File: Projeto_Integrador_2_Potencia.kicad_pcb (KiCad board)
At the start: 2 copper layers, 150 x 100 mm, 17 parts, among them J10 Borne_CMD_Interface, J2 Vi 24V, J3 Vo 48V, J4 INA219_01x02_Socket_3.5mm, J5 INA219_01x06_Socket_2.55mm, J7 Display_01x04_Socket, J9 PWM_Connector, Q1 IRF740, U1 ESP32-DEVKIT-V1

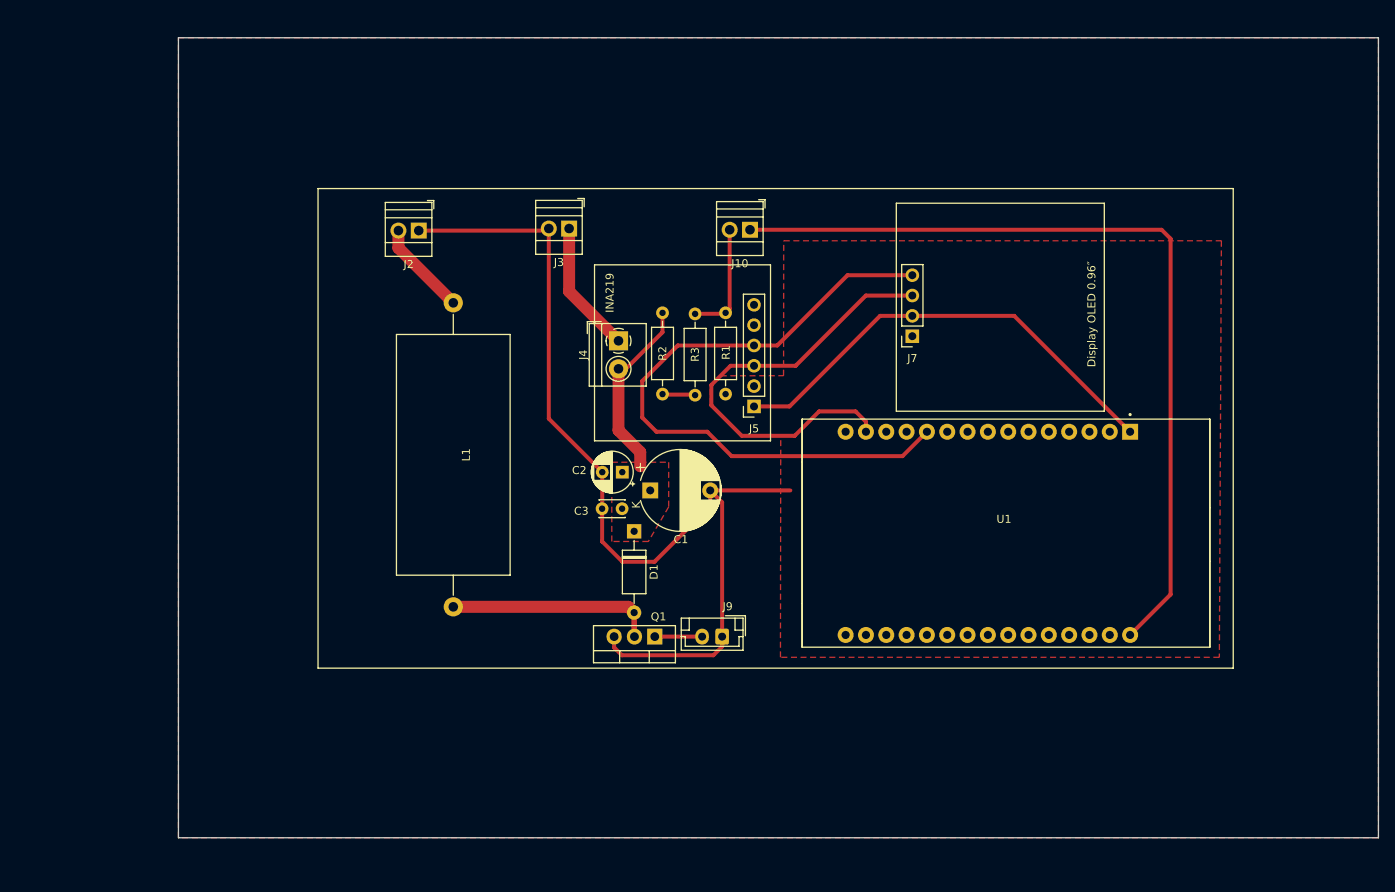
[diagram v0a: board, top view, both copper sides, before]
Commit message: Mudanças após primeira manufatura
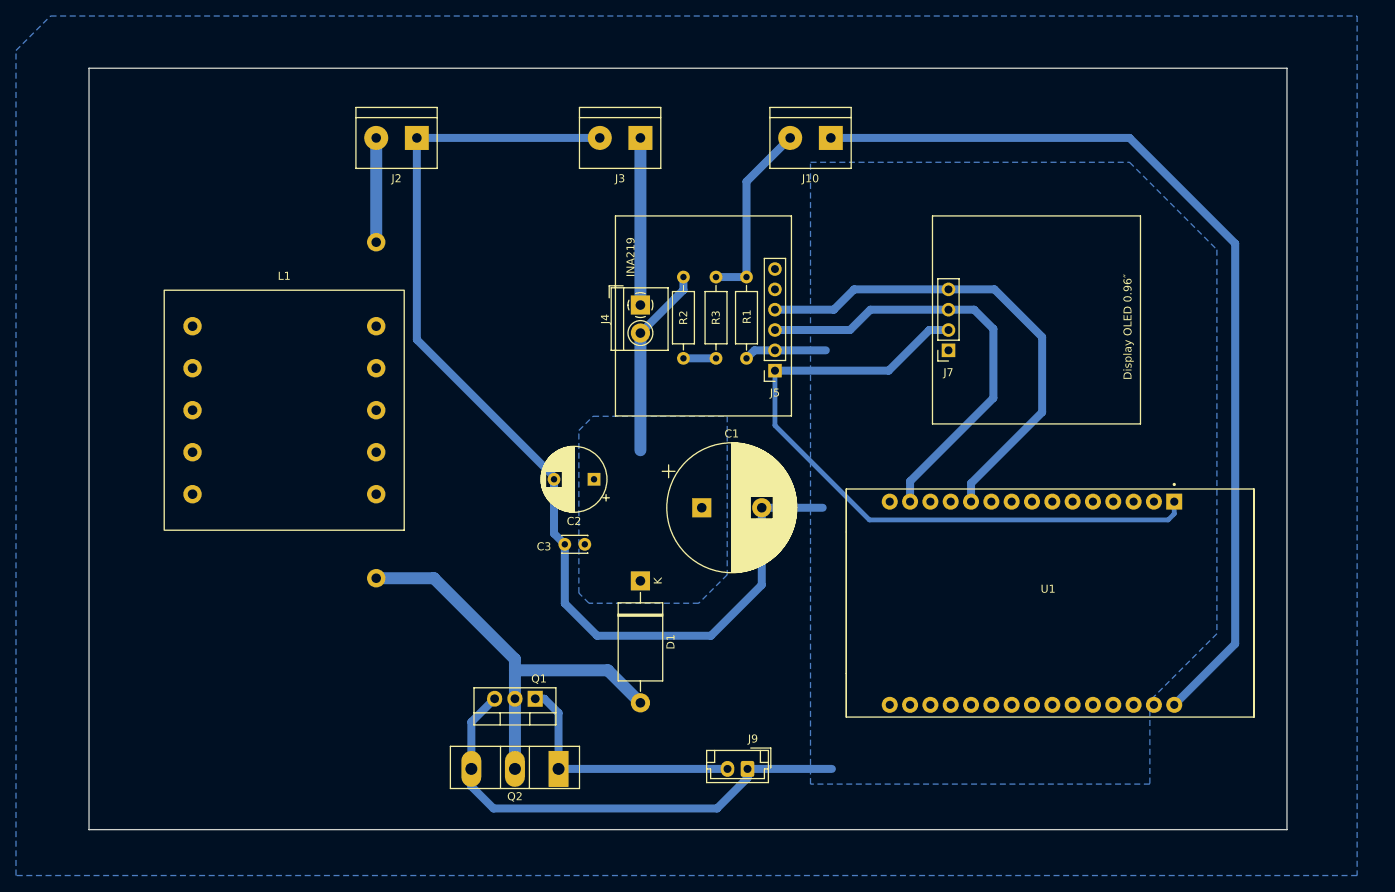
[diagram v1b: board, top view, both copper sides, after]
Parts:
- added Q2: 47N60, Package_TO_SOT_THT:TO-247-3_Vertical, F.Cu at (112.0, 137.3)
- C1: footprint Capacitor_THT:CP_Radial_D10.0mm_P7.50mm -> Capacitor_THT:CP_Radial_D16.0mm_P7.50mm
- C2: footprint Capacitor_THT:CP_Radial_D5.0mm_P2.50mm -> Capacitor_THT:CP_Radial_D8.0mm_P5.00mm
- D1: value ~ -> Diodo Schottky; footprint Diode_THT:D_A-405_P10.16mm_Horizontal -> Diode_THT:D_DO-27_P15.24mm_Horizontal
- J10, J2, J3: footprint TerminalBlock:TerminalBlock_Xinya_XY308-2.54-2P_1x02_P2.54mm_Horizontal -> TerminalBlock:TerminalBlock_bornier-2_P5.08mm
- L1: footprint Inductor_THT:L_Axial_L29.9mm_D14.0mm_P38.00mm_Horizontal_Vishay_IHA-105 -> Integrador_2:Indutor_Integrador_2
- moved L1 25.0 mm to (77.7, 92.5), turned to 180 degrees
- moved J9 16.8 mm to (135.6, 137.3)
- moved Q1 16.8 mm to (109.1, 128.5)
- moved J10 15.3 mm to (146.1, 58.4)
- moved J3 14.4 mm to (122.2, 58.4)
- moved J2 11.6 mm to (94.3, 58.4)
- moved U1 10.3 mm to (173.5, 116.6)
- moved C1 6.79 mm to (129.9, 104.6)
- moved C3 6.45 mm to (115.3, 109.2)
- moved D1 6.25 mm to (122.2, 113.8)
- moved R3 5.30 mm to (131.7, 86.0)
- moved J4 5.24 mm to (122.2, 79.3)
- moved R1 5.18 mm to (135.5, 75.8)
- moved R2 5.18 mm to (127.6, 75.8)
- moved J5 5.18 mm to (139.1, 87.5)
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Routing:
- net GND: track 123.5 -> 206.3 mm
- net 3V3: track 57.6 -> 87.3 mm
- net pwm: track 5.92 -> 31.8 mm
- net Net-(D1-A): track 27.4 -> 52.6 mm
- net I2C_Sda: track 82.6 -> 61.2 mm
- net 8V: track 104.7 -> 116.8 mm
- net 5.2V_feedback: track 14.5 -> 23.5 mm
- net INA_Vin+: track 16.6 -> 20.9 mm
- net Net-(J2-Pin_2): track 11.9 -> 13.0 mm
- net I2C_Scl: track 56.2 -> 55.3 mm
- net INA_Vin-: track 23.1 -> 23.9 mm
- added copper zone on B.Cu, net (none)
- added copper zone on B.Cu, net GND
- added copper zone on B.Cu, net INA_Vin-
- removed copper zone on F.Cu, net (none)
- removed copper zone on F.Cu, net GND
- removed copper zone on F.Cu, net INA_Vin-
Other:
- board size 150 x 100 mm -> 149.7 x 95.2 mm
